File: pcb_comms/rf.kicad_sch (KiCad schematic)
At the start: 25 parts, among them IC4 BGS12WN6E6329XTSA1

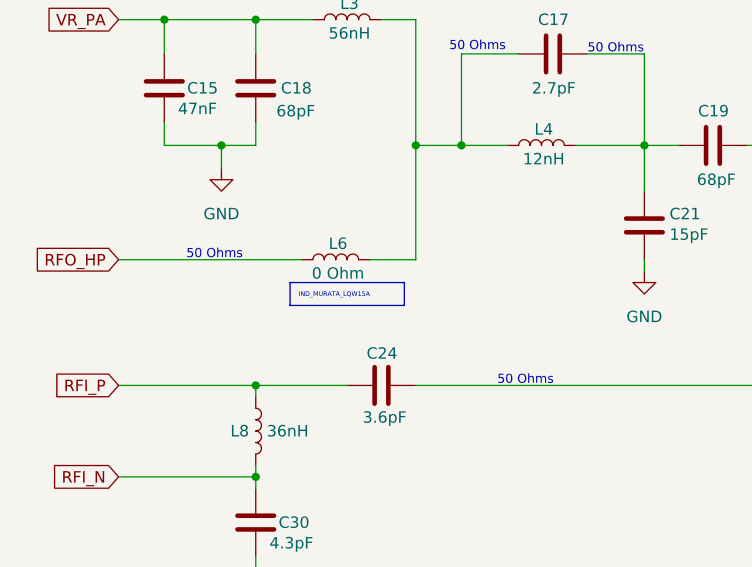
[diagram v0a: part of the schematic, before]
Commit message: Version 1.0. No DRA yet
From now on I will make the connections for IIS and then adapt it for the club
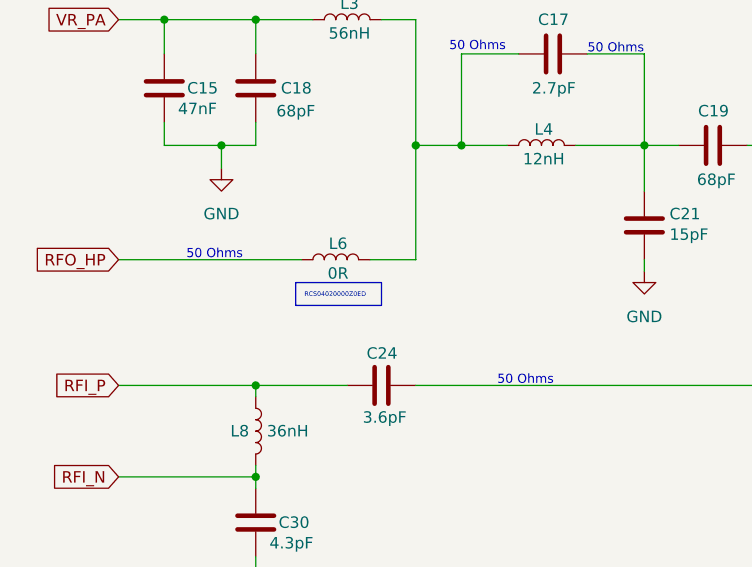
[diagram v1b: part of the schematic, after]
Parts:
- L6: value 0 Ohm -> 0R
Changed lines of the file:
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@@
 		)
 	)
-	(text_box "IND_MURATA_LQW15A"
+	(text_box "RCS04020000Z0ED"
 		(exclude_from_sim no)
-		(at 68.58 73.66 0)
-		(size 12.7 2.54)
+		(at 69.215 73.66 0)
+		(size 9.525 2.54)
 		(margins 0.9525 0.9525 0.9525 0.9525)
 		(stroke
@@
 			)
 		)
-		(property "Value" "0 Ohm"
+		(property "Value" "0R"
 			(at 73.914 72.644 90)
 			(effects
